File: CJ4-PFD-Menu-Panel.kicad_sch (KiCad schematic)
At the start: 25 parts

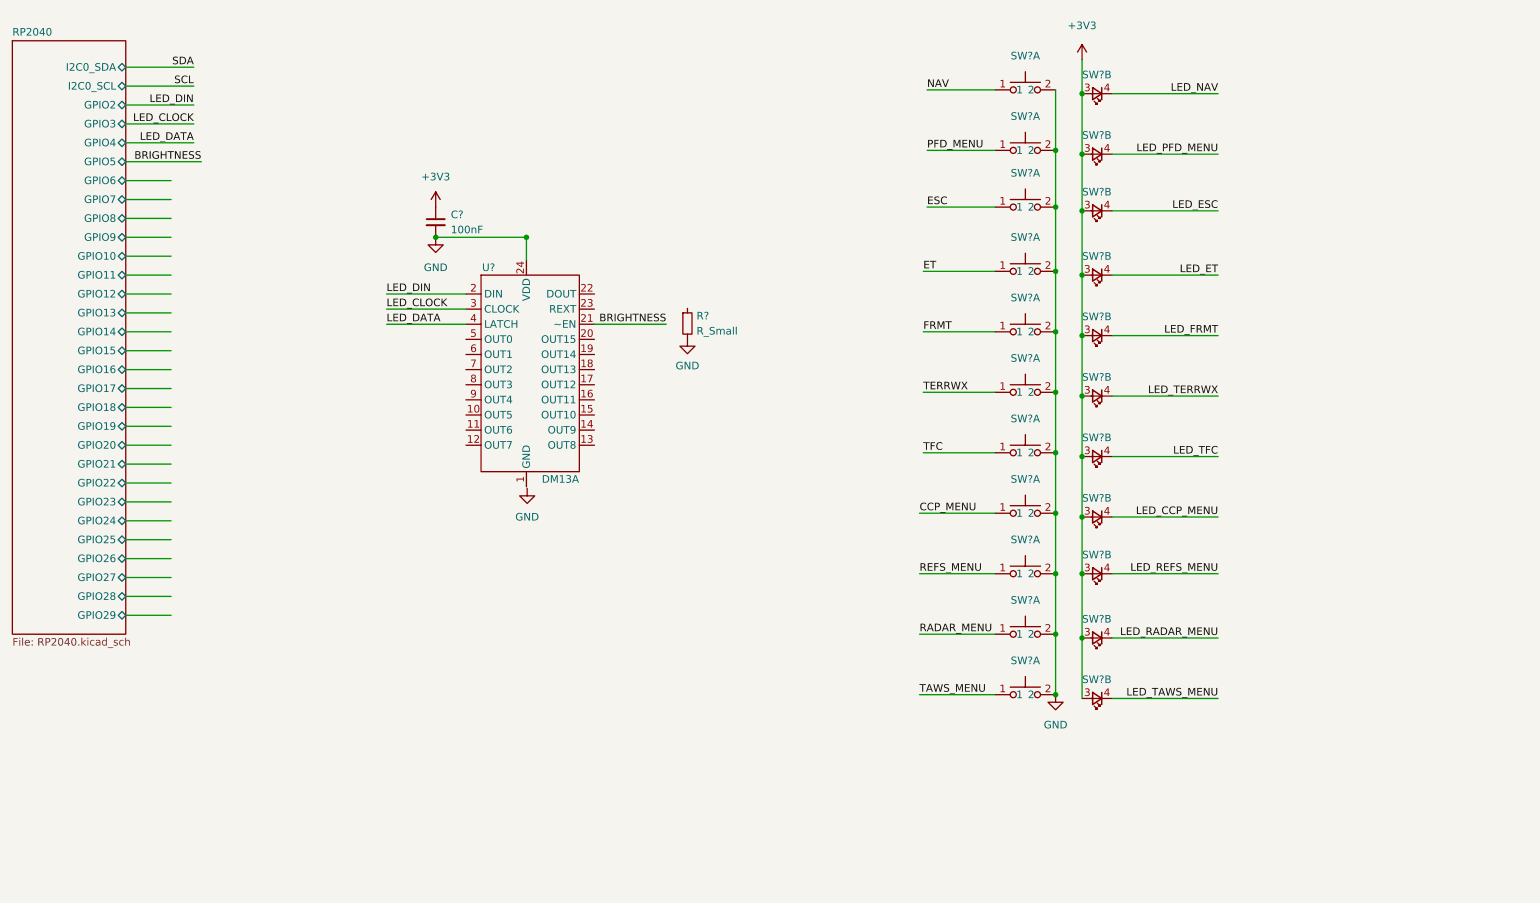
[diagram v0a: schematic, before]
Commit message: Initial schematic complete
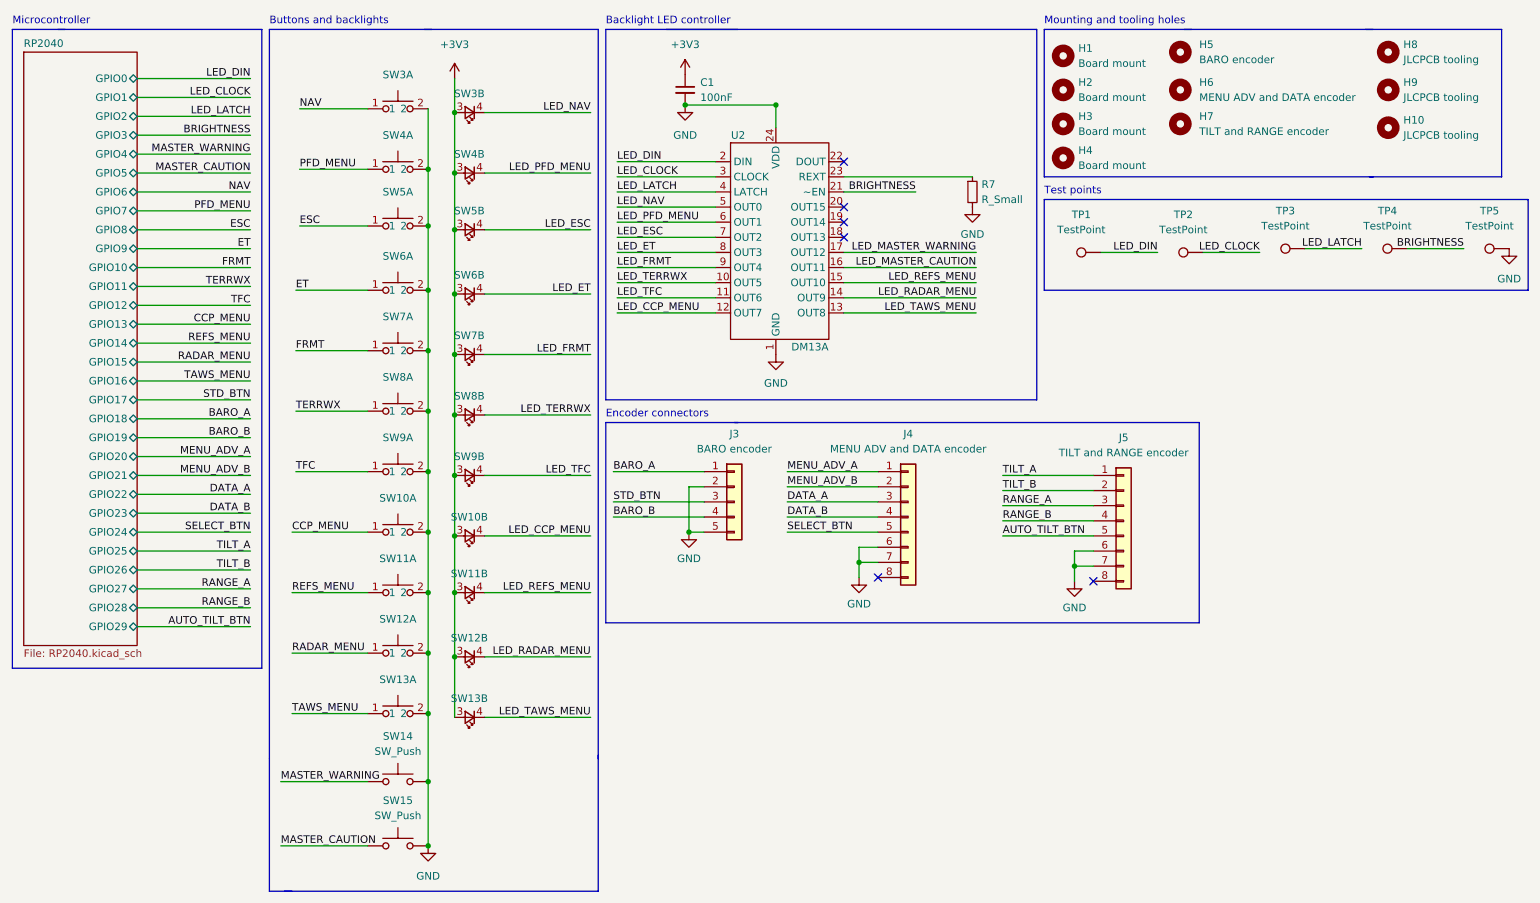
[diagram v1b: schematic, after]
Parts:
- added H1, H2, H3, H4: Board mount, MountingHole:MountingHole_3.2mm_M3, symbol Mechanical:MountingHole
- added H10, H8, H9: JLCPCB tooling, Custom_Footprints:JLCPCB_Tooling_Hole, symbol Mechanical:MountingHole
- added H5: BARO encoder, Custom_Footprints:EN11-HSM1BF20 panel mount, symbol Mechanical:MountingHole
- added H6: MENU ADV and DATA encoder, Custom_Footprints:EC11E-BB24C03_PM, symbol Mechanical:MountingHole
- added H7: TILT and RANGE encoder, Custom_Footprints:EC11E-BB24C03_PM, symbol Mechanical:MountingHole
- added J3: BARO encoder, Connector_JST:JST_XH_B5B-XH-A_1x05_P2.50mm_Vertical, symbol Connector_Generic:Conn_01x05
- added J4: MENU ADV and DATA encoder, Connector_JST:JST_XH_B8B-XH-A_1x08_P2.50mm_Vertical, symbol Connector_Generic:Conn_01x08
- added J5: TILT and RANGE encoder, Connector_JST:JST_XH_B8B-XH-A_1x08_P2.50mm_Vertical, symbol Connector_Generic:Conn_01x08
- added SW14, SW15: SW_Push, symbol Switch:SW_Push
- added TP1, TP2, TP3, TP4, TP5: TestPoint, TestPoint:TestPoint_Keystone_5000-5004_Miniature, symbol Connector:TestPoint
- C1: renamed from C?; footprint (none) -> Custom_Footprints:Perfect_0402
- R7: renamed from R?; footprint (none) -> Custom_Footprints:Perfect_0402
- gave numbers to parts that had none: 12
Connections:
- net BRIGHTNESS: now also TP4.1
- net GND: now also U2.1 (GND), J3.2 (Pin_2), J3.5 (Pin_5), J4.6 (Pin_6), J4.7 (Pin_7), J5.6 (Pin_6), J5.7 (Pin_7), SW14.2, SW15.2, TP5.1
- net LED_CCP_MENU: now also U2.12 (OUT7)
- net LED_CLOCK: now also TP2.1
- net LED_DIN: now also TP1.1
- net LED_ESC: now also U2.7 (OUT2)
- net LED_ET: now also U2.8 (OUT3)
- net LED_FRMT: now also U2.9 (OUT4)
- net LED_NAV: now also U2.5 (OUT0)
- net LED_PFD_MENU: now also U2.6 (OUT1)
- net LED_RADAR_MENU: now also U2.14 (OUT9)
- net LED_REFS_MENU: now also U2.15 (OUT10)
- net LED_TAWS_MENU: now also U2.13 (OUT8)
- net LED_TERRWX: now also U2.10 (OUT5)
- net LED_TFC: now also U2.11 (OUT6)
- net at R7.1: now also U2.23 (REXT)
- net LED_MASTER_CAUTION: now reaches U2.16 (OUT11)
- net LED_MASTER_WARNING: now reaches U2.17 (OUT12)
- net LED_DATA renamed LED_LATCH
- net LED_LATCH: now also TP3.1
- new net AUTO_TILT_BTN: J5.5 (Pin_5)
- new net BARO_A: J3.1 (Pin_1)
- new net BARO_B: J3.4 (Pin_4)
- new net DATA_A: J4.3 (Pin_3)
- new net DATA_B: J4.4 (Pin_4)
- new net MASTER_CAUTION: SW15.1
- new net MASTER_WARNING: SW14.1
- new net MENU_ADV_A: J4.1 (Pin_1)
- new net MENU_ADV_B: J4.2 (Pin_2)
- new net RANGE_A: J5.3 (Pin_3)
- new net RANGE_B: J5.4 (Pin_4)
- new net SELECT_BTN: J4.5 (Pin_5)
- new net STD_BTN: J3.3 (Pin_3)
- new net TILT_A: J5.1 (Pin_1)
- new net TILT_B: J5.2 (Pin_2)
- no-connect marks 0 -> 6
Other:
- sheet RP2040 ports: added GPIO0, GPIO1; removed I2C0_SCL, I2C0_SDA
- note added: "Backlight LED controller"
- note added: "Buttons and backlights"
- note added: "Encoder connectors"
- note added: "Microcontroller"
- note added: "Mounting and tooling holes"
- note added: "Test points"
- moved on the sheet: C1, R7, SW10A, SW10B, SW11A, SW11B, SW12A, SW12B, SW13A, SW13B, SW3A, SW3B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
